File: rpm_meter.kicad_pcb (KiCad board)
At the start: 2 copper layers, 122.3 x 96.7 mm, 118 parts, among them IC1 SN74LV1T34DCKR, IC6 TPS566247DRLR, J1 Conn_01x05_Pin, Q1 BC846, Q12 BC846, Q13 AO3423, Q14 BC846, Q15 BC846, Q16 BC846, U1 M24C02-RMN, U2 STM32C031C6Tx, U3 74LVC1G123, U4 TLV1117-33, Y1 8

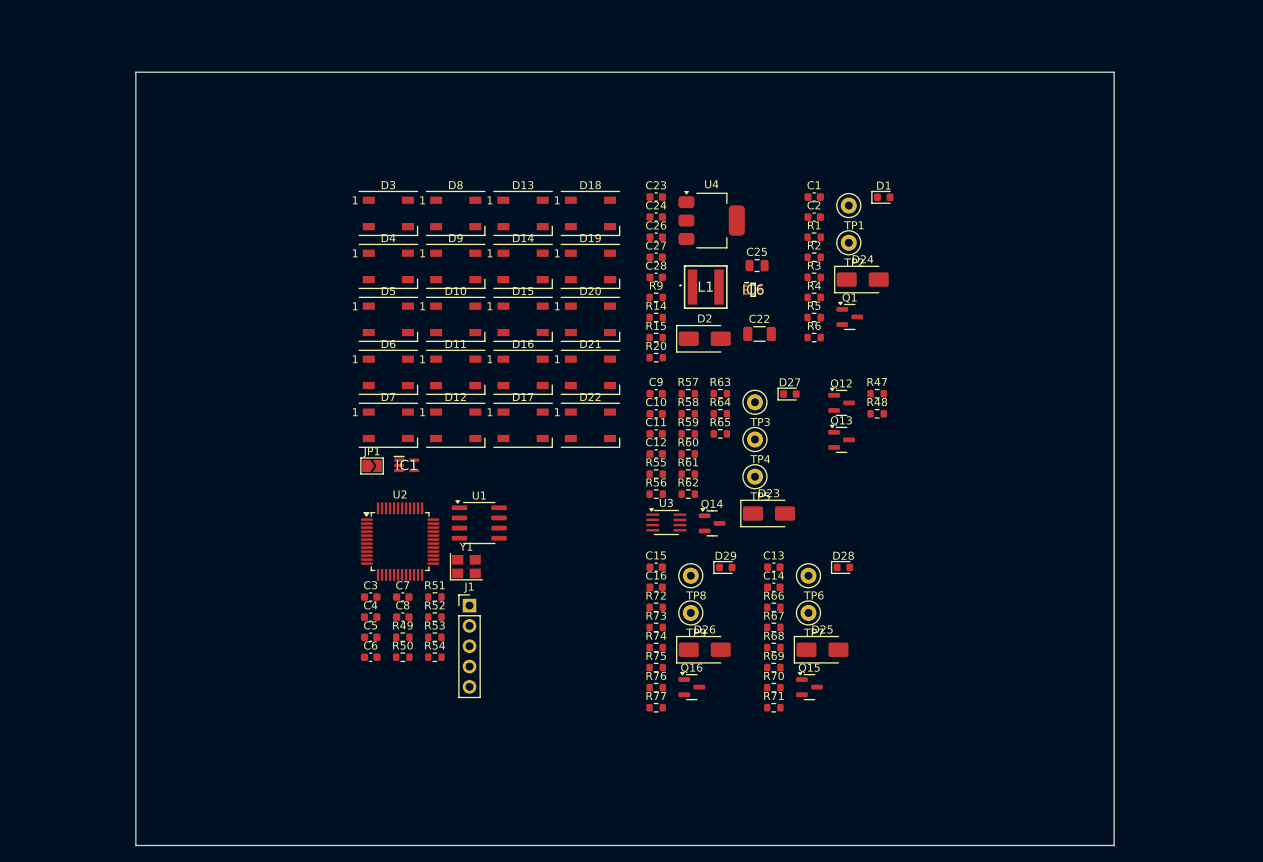
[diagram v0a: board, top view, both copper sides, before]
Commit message: Placed footprints v1.0
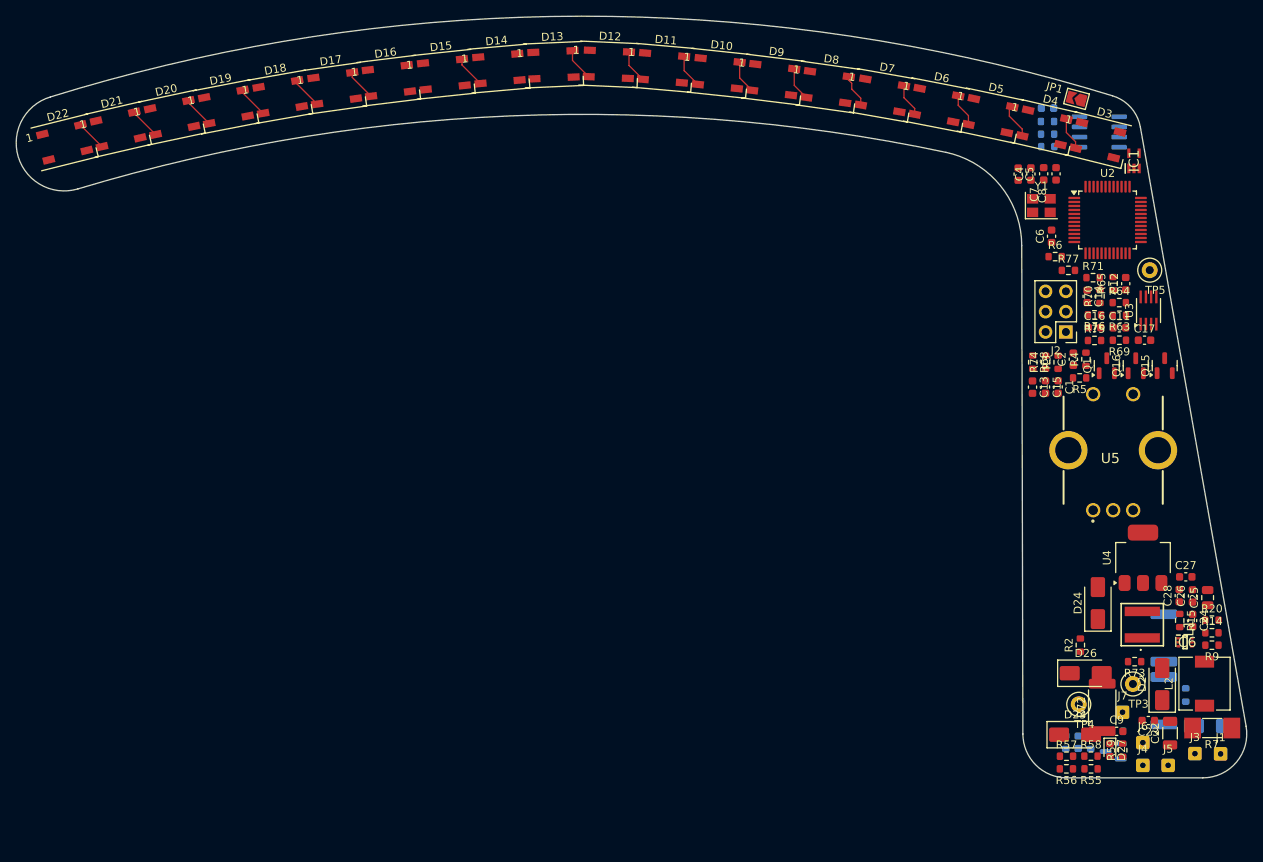
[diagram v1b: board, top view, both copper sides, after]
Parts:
- removed D1, D28, D29: D_Schottky, Diode_SMD:D_0603_1608Metric
- removed Q12: BC846, Package_TO_SOT_SMD:SOT-23
- removed Q13: AO3423, Package_TO_SOT_SMD:SOT-23
- removed R47: 1k, Resistor_SMD:R_0603_1608Metric
- removed R48, R49, R50, R51: 10k, Resistor_SMD:R_0603_1608Metric
- removed TP1, TP2, TP6, TP7, TP8, TP9: TestPoint, TestPoint:TestPoint_Loop_D1.80mm_Drill1.0mm_Beaded
- added C17: 100n, Capacitor_SMD:C_0603_1608Metric, F.Cu at (209.2, 70.2)
- added J2: Conn_2Rows-05Pins, Connector_PinHeader_2.54mm:PinHeader_2x03_P2.54mm_Vertical, F.Cu at (199.3, 69.1)
- added J3: Conn_01x01_Socket, Connector_Wire:SolderWire-0.15sqmm_1x01_D0.5mm_OD1.5mm, F.Cu at (215.5, 121.8)
- added J4: Conn_01x01_Socket, Connector_Wire:SolderWire-0.15sqmm_1x01_D0.5mm_OD1.5mm, F.Cu at (209.0, 123.3)
- added J5: Conn_01x01_Socket, Connector_Wire:SolderWire-0.15sqmm_1x01_D0.5mm_OD1.5mm, F.Cu at (212.1, 123.3)
- added J6: Conn_01x01_Socket, Connector_Wire:SolderWire-0.15sqmm_1x01_D0.5mm_OD1.5mm, F.Cu at (209.0, 120.5)
- added J7: Conn_01x01_Socket, Connector_Wire:SolderWire-0.15sqmm_1x01_D0.5mm_OD1.5mm, F.Cu at (206.4, 116.7)
- added L2: 6,8u, Inductor_SMD:L_6.3x6.3_H3, F.Cu at (216.7, 113.1)
- added R7: 0,1, Resistor_SMD:R_MELF_MMB-0207, F.Cu at (217.6, 118.6)
- added U5: PEC11R-4225F-S0024, Library_local:PEC12R-4XXXF-SXXXX_1, F.Cu at (205.2, 83.9)
- C10, C3, D25, Q14, R52, R53, R54, R60, R61, R62, R67, U1: moved to B.Cu
- J1: value Conn_01x05_Pin -> Conn_01x01_Socket; footprint Connector_PinHeader_2.54mm:PinHeader_1x05_P2.54mm_Vertical -> Connector_Wire:SolderWire-0.15sqmm_1x01_D0.5mm_OD1.5mm
- R1, R66: footprint Resistor_SMD:R_0603_1608Metric -> Resistor_SMD:R_2512_6332Metric; moved to B.Cu
- R72: footprint Resistor_SMD:R_0603_1608Metric -> Resistor_SMD:R_2512_6332Metric
- moved C3 104.4 mm to (197.0, 41.1)
- moved R54 101.7 mm to (197.0, 42.8), turned to 180 degrees
- moved C6 100.1 mm to (197.6, 57.2), turned to 90 degrees
- moved C5 99.5 mm to (193.4, 49.4), turned to -90 degrees
- moved C4 99.4 mm to (195.0, 49.4), turned to 90 degrees
- moved JP1 99.3 mm to (200.7, 40.0), turned to 165 degrees
- moved R53 99.1 mm to (197.1, 44.4), turned to 180 degrees
- moved C8 98.7 mm to (198.1, 49.4), turned to 90 degrees
- moved IC1 98.6 mm to (207.9, 47.7), turned to 90 degrees
- moved U2 97.1 mm to (204.6, 55.1)
- moved R52 96.6 mm to (197.1, 46.0), turned to 180 degrees
- moved C7 96.0 mm to (196.6, 49.4), turned to 90 degrees
- moved J1 95.7 mm to (218.7, 121.9)
- moved U1 91.6 mm to (203.5, 44.1), turned to 180 degrees
- moved C23 89.8 mm to (209.6, 117.7), turned to 180 degrees
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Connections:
- C1 pad 1: Net-(D1-K) -> Net-(D24-A2)
- C13 pad 1: Net-(D28-K) -> Net-(D25-A2)
- C15 pad 1: Net-(D29-K) -> Net-(D26-A2)
- C22 pad 1: +12V -> Net-(D2-A2)
- C23 pad 1: +12V -> Net-(D2-A2)
- D2 pad 2: +12V -> Net-(D2-A2)
- D24 pad 2: Net-(D1-A) -> Net-(D24-A2)
- IC6 pad 1: +12V -> Net-(IC6-VIN)
- J1 pad 1: /mcu/TMS -> +12V
- R1 pad 2: Net-(D1-A) -> Net-(D24-A2)
- R2 pad 2: Net-(D1-K) -> Net-(D24-A2)
- R3 pad 1: Net-(D1-K) -> Net-(D24-A2)
- R67 pad 2: Net-(D28-K) -> Net-(D25-A2)
- R68 pad 1: Net-(D28-K) -> Net-(D25-A2)
- R73 pad 2: Net-(D29-K) -> Net-(D26-A2)
- R74 pad 1: Net-(D29-K) -> Net-(D26-A2)
- R9 pad 1: +12V -> Net-(IC6-VIN)
- U1 pad 1: Net-(U1-E0) -> GND
- U1 pad 2: Net-(U1-E1) -> GND
- U1 pad 3: Net-(U1-E2) -> GND
- U2 pad 39: /led_pwm_5v/led_pwm_signal -> /mcu/led_pwm_out_3v3
- U3 pad 4: unconnected-(U3B-GND-Pad4) -> GND
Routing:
- net Net-(D4-DOUT): track 0.00 -> 4.45 mm
- net Net-(D10-DOUT): track 0.00 -> 4.21 mm
- net Net-(D8-DOUT): track 0.00 -> 4.19 mm
- net Net-(D10-DIN): track 0.00 -> 4.16 mm
- net Net-(D7-DOUT): track 0.00 -> 4.15 mm
- net Net-(D3-DOUT): track 0.00 -> 4.13 mm
- net Net-(D11-DOUT): track 0.00 -> 4.13 mm
- net Net-(D6-DOUT): track 0.00 -> 4.12 mm
- net Net-(D5-DOUT): track 0.00 -> 4.11 mm
- net Net-(D12-DOUT): track 0.00 -> 4.09 mm
- net Net-(D14-DOUT): track 0.00 -> 4.00 mm
- net Net-(D17-DOUT): track 0.00 -> 3.98 mm
- net Net-(D18-DOUT): track 0.00 -> 3.96 mm
- net Net-(D19-DOUT): track 0.00 -> 3.95 mm
- net Net-(D16-DOUT): track 0.00 -> 3.95 mm
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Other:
- board size 122.3 x 96.7 mm -> 153.8 x 95.2 mm
